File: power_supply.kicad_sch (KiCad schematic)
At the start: 24 parts, among them U3 ST1S10PHR, U4 ST1S09IPUR

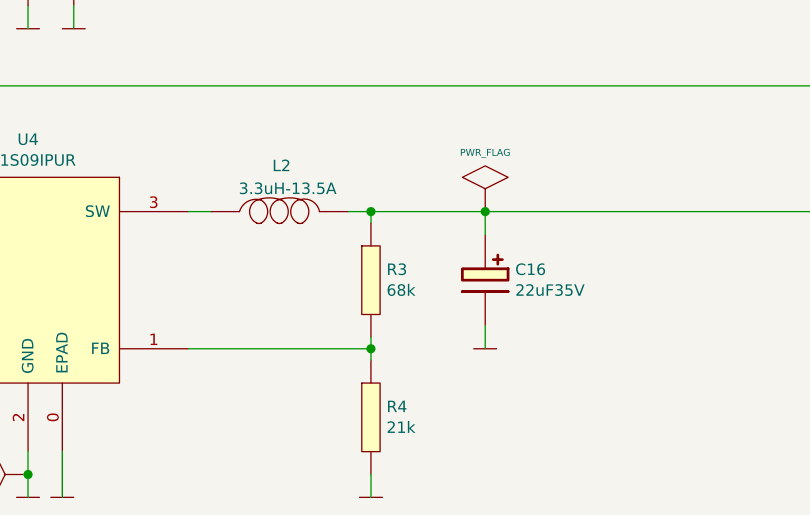
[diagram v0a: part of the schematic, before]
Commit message: Gerbers created, BOM, CPL
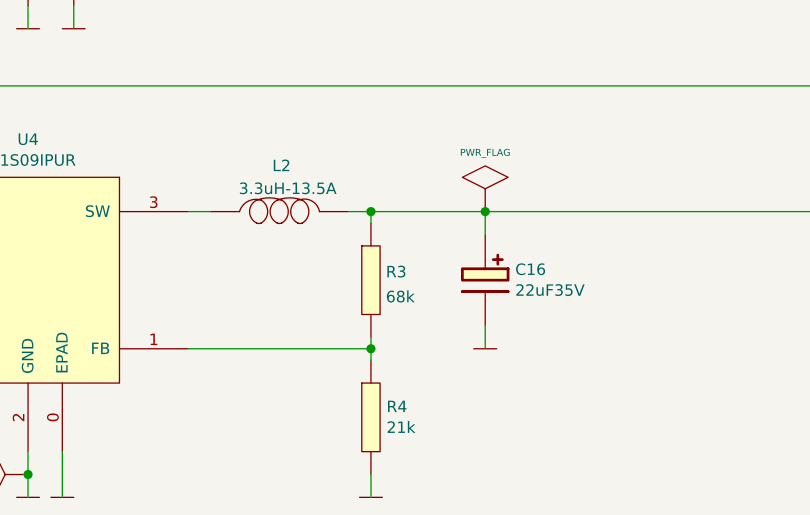
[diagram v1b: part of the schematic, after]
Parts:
- R2, R6: Price@1pc (none) -> 0,07119
- R3: Developer (none) -> MW; Field11 MW -> (none)
- R4: Price@1pc (none) -> 0,05002
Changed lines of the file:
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@@
+      (effects (font (size 1.27 1.27)) hide)
+    )
+    (property "Price@1pc" "0,07119" (id 14) (at 266.7 125.73 0)
       (effects (font (size 1.27 1.27)) hide)
     )
@@
       (effects (font (size 1.27 1.27)) hide)
     )
-    (property "Datasheet" "Resistors/Smd_0603/Components_Documentation/Vishay_Resistors_SM0603.pdf" (id 3) (at 262.89 121.92 0)
+    (property "Datasheet" "https://www.tme.eu/Document/b315665a56acbc42df513c99b390ad98/ROYALOHM-THICKFILM.pdf" (id 3) (at 262.89 121.92 0)
       (effects (font (size 1.27 1.27)) hide)
     )
@@
     )
     (property "LCSC Part #(optional)" "C234435" (id 13) (at 186.69 114.3 0)
+      (effects (font (size 1.27 1.27)) hide)
+    )
+    (property "Price@1pc" "0,07119" (id 14) (at 186.69 114.3 0)
       (effects (font (size 1.27 1.27)) hide)
     )
@@
       (effects (font (size 1.27 1.27)) hide)
     )
+    (property "Price@1pc" "0,05002" (id 14) (at 251.46 182.88 0)
+      (effects (font (size 1.27 1.27)) hide)
+    )
     (pin "1")
     (pin "2")
@@
     )
     (property "Package" "7.2 mm x 6.65 mm x 3 mm" (id 12) (at 241.3 160.02 0)
-      (effects (font (size 1.27 1.27)) hide)
-    )
-    (pin "1")
-    (pin "2")
-  )
-  (symbol (lib_id "Resistors_Smd0603:68k") (at 251.46 167.64 0) (unit 1)
-    (in_bom yes) (on_board yes)
-    (property "Reference" "R3" (id 0) (at 253.1872 166.4716 0)
-      (effects (font (size 1.27 1.27)) (justify left))
-    )
-    (property "Value" "68k" (id 1) (at 253.1872 168.783 0)
-      (effects (font (size 1.27 1.27)) (justify left))
-    )
-    (property "Footprint" "Resistor_Smd_0603:68k_0603" (id 2) (at 251.46 179.07 0)
-      (effects (font (size 1.27 1.27)) hide)
-    )
-    (property "Datasheet" "Resistors/Smd_0603/Components_Documentation/Vishay_Resistors_SM0603.pdf" (id 3) (at 251.46 179.07 0)
-      (effects (font (size 1.27 1.27)) hide)
-    )
-    (property "Manufacturer" "ROYAL OHM" (id 4) (at 251.46 167.64 0)
-      (effects (font (size 1.27 1.27)) hide)
-    )
-    (property "Manufacturer Part Number" "0603SAF6802T5E" (id 5) (at 251.46 167.64 0)
-      (effects (font (size 1.27 1.27)) hide)
-    )
-    (property "Supplier" "TME" (id 6) (at 251.46 167.64 0)
-      (effects (font (size 1.27 1.27)) hide)
-    )
-    (property "Supplier Part Number" "SMD0603-68K-1%" (id 7) (at 251.46 167.64 0)
-      (effects (font (size 1.27 1.27)) hide)
-    )
-    (property "URL" "https://www.tme.eu/pl/details/smd0603-68k-1%2525/rezystory-smd-0603/royal-ohm/0603saf6802t5e/" (id 8) (at 251.46 167.64 0)
-      (effects (font (size 1.27 1.27)) hide)
-    )
-    (property "Price@1pc" "0,04693" (id 9) (at 251.46 167.64 0)
-      (effects (font (size 1.27 1.27)) hide)
-    )
-    (property "Price@1000pcs" "0,01269" (id 10) (at 251.46 167.64 0)
-      (effects (font (size 1.27 1.27)) hide)
-    )
-    (property "Field11" "MW" (id 11) (at 251.46 167.64 0)
-      (effects (font (size 1.27 1.27)) hide)
-    )
-    (property "Package" "0603" (id 12) (at 251.46 167.64 0)
-      (effects (font (size 1.27 1.27)) hide)
-    )
-    (property "LCSC Part #(optional)" "C160055" (id 13) (at 251.46 167.64 0)
       (effects (font (size 1.27 1.27)) hide)
     )
@@
     (pin "1")
   )
+  (symbol (lib_id "Resistors_Smd0603:68k") (at 251.46 167.64 0) (unit 1)
+    (in_bom yes) (on_board yes) (fields_autoplaced)
+    (property "Reference" "R3" (id 0) (at 253.111 166.7315 0)
+      (effects (font (size 1.27 1.27)) (justify left))
+    )
+    (property "Value" "68k" (id 1) (at 253.111 169.5066 0)
+      (effects (font (size 1.27 1.27)) (justify left))
+    )
+    (property "Footprint" "Resistor_Smd_0603:68k_0603" (id 2) (at 251.46 179.07 0)
+      (effects (font (size 1.27 1.27)) hide)
+    )
+    (property "Datasheet" "https://www.tme.eu/Document/4f50d320a6ddacb273098f84373b6259/rezystor-smd.pdf" (id 3) (at 251.46 179.07 0)
+      (effects (font (size 1.27 1.27)) hide)
+    )
+    (property "Manufacturer" "ROYAL OHM" (id 4) (at 251.46 167.64 0)
+      (effects (font (size 1.27 1.27)) hide)
+    )
+    (property "Manufacturer Part Number" "0603SAF6802T5E" (id 5) (at 251.46 167.64 0)
+      (effects (font (size 1.27 1.27)) hide)
+    )
+    (property "Supplier" "TME" (id 6) (at 251.46 167.64 0)
+      (effects (font (size 1.27 1.27)) hide)
+    )
+    (property "Supplier Part Number" "SMD0603-68K-1%" (id 7) (at 251.46 167.64 0)
+      (effects (font (size 1.27 1.27)) hide)
+    )
+    (property "URL" "https://www.tme.eu/pl/details/smd0603-68k-1%2525/rezystory-smd-0603/royal-ohm/0603saf6802t5e/" (id 8) (at 251.46 167.64 0)
+      (effects (font (size 1.27 1.27)) hide)
+    )
+    (property "Price@1pc" "0,04693" (id 9) (at 251.46 167.64 0)
+      (effects (font (size 1.27 1.27)) hide)
+    )
+    (property "Price@1000pcs" "0,01269" (id 10) (at 251.46 167.64 0)
+      (effects (font (size 1.27 1.27)) hide)
+    )
+    (property "Developer" "MW" (id 11) (at 251.46 167.64 0)
+      (effects (font (size 1.27 1.27)) hide)
+    )
+    (property "Package" "0603" (id 12) (at 251.46 167.64 0)
+      (effects (font (size 1.27 1.27)) hide)
+    )
+    (property "LCSC Part #(optional)" "C160055" (id 13) (at 251.46 167.64 0)
+      (effects (font (size 1.27 1.27)) hide)
+    )
+    (pin "1")
+    (pin "2")
+  )
   (symbol (lib_id "power:GND_NO_GLOBAL") (at 217.17 191.77 0) (unit 1)
